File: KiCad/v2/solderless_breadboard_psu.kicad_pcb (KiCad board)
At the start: 4 copper layers, 53 x 51 mm, 78 parts, among them IC201 TPS63000DRCR, IC202 TPS63000DRCR, IC301 CP2102N-A02-GQFN24R, J201 Conn_01x02_Pin, J202 Conn_01x03_Pin, J203 Conn_02x03_Odd_Even, J204 Conn_01x03_Pin, J205 Conn_02x03_Odd_Even, J301 Conn_01x09_Pin, J302 Conn_01x09_Pin, J303 Conn_01x06_Pin, J304 USB_C_Receptacle_USB2.0_16P, J305 Conn_01x03_Pin, U301 USBLC6-2SC6

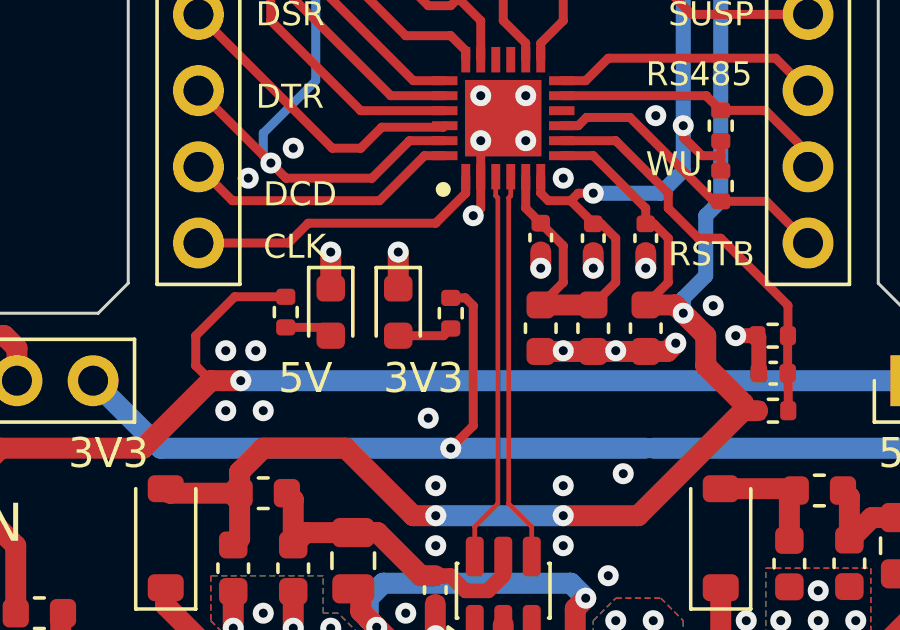
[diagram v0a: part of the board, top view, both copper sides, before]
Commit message: BOM updates
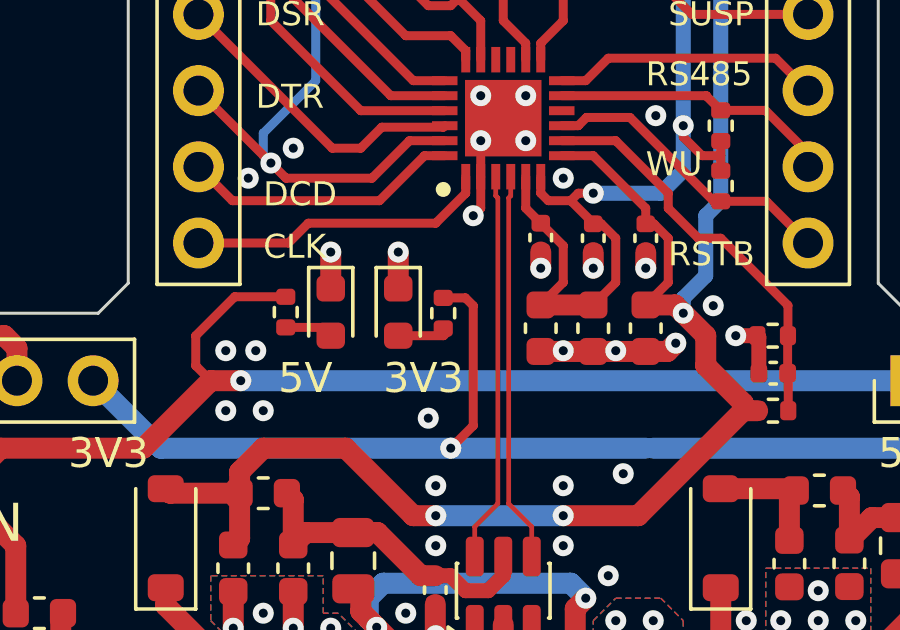
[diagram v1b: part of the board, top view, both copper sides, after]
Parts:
- R203: value 900kR -> 910kR
- moved R205 0.25 mm to (74.5, 78.5)
